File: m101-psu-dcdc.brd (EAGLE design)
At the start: 100 x 50 mm, 49 parts, among them U1 SCREW-M2X8, U2 SCREW-M2X8, U3 NUT-M2-SELFLOCK, U4 NUT-M2-SELFLOCK, U5 FX2-20P-1.27DS, U6 SHHN000A3CL41Z, U7 G3VM-62C1, U8 ERM1-5MM

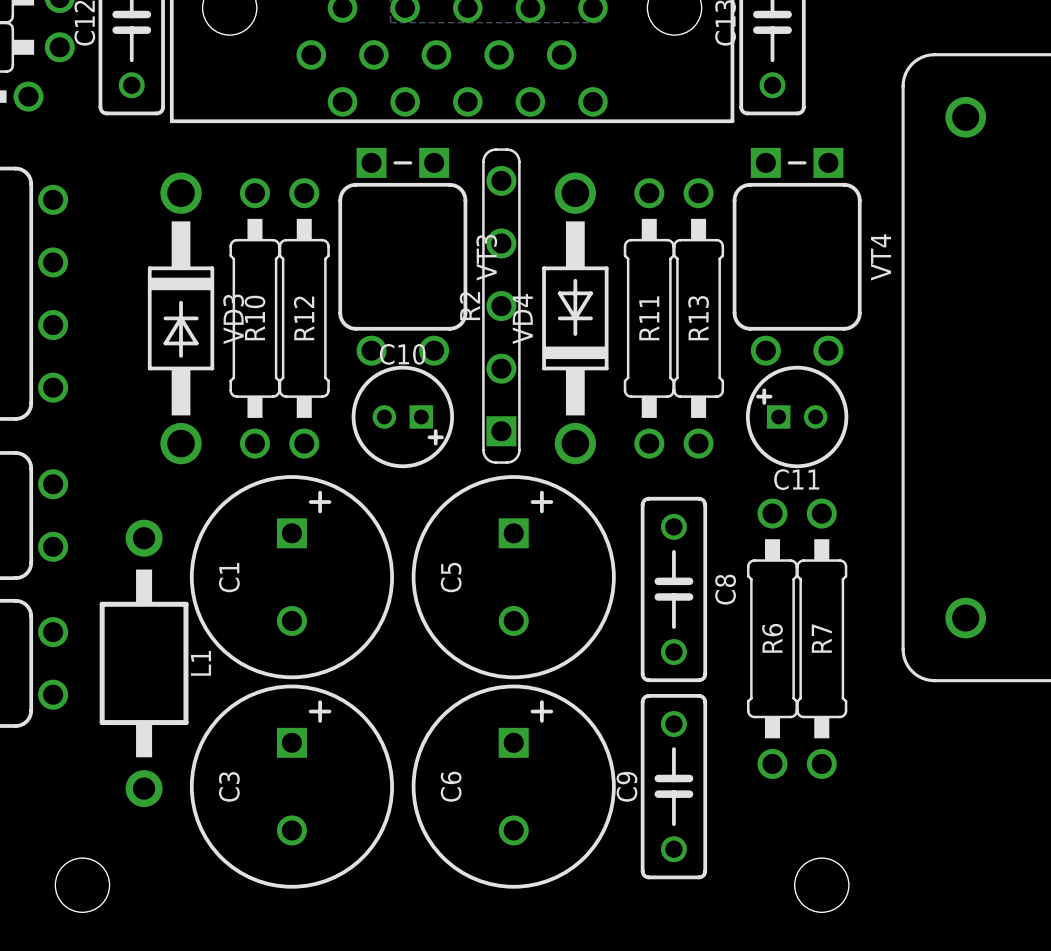
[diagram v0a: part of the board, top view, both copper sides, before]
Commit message: M101c Update
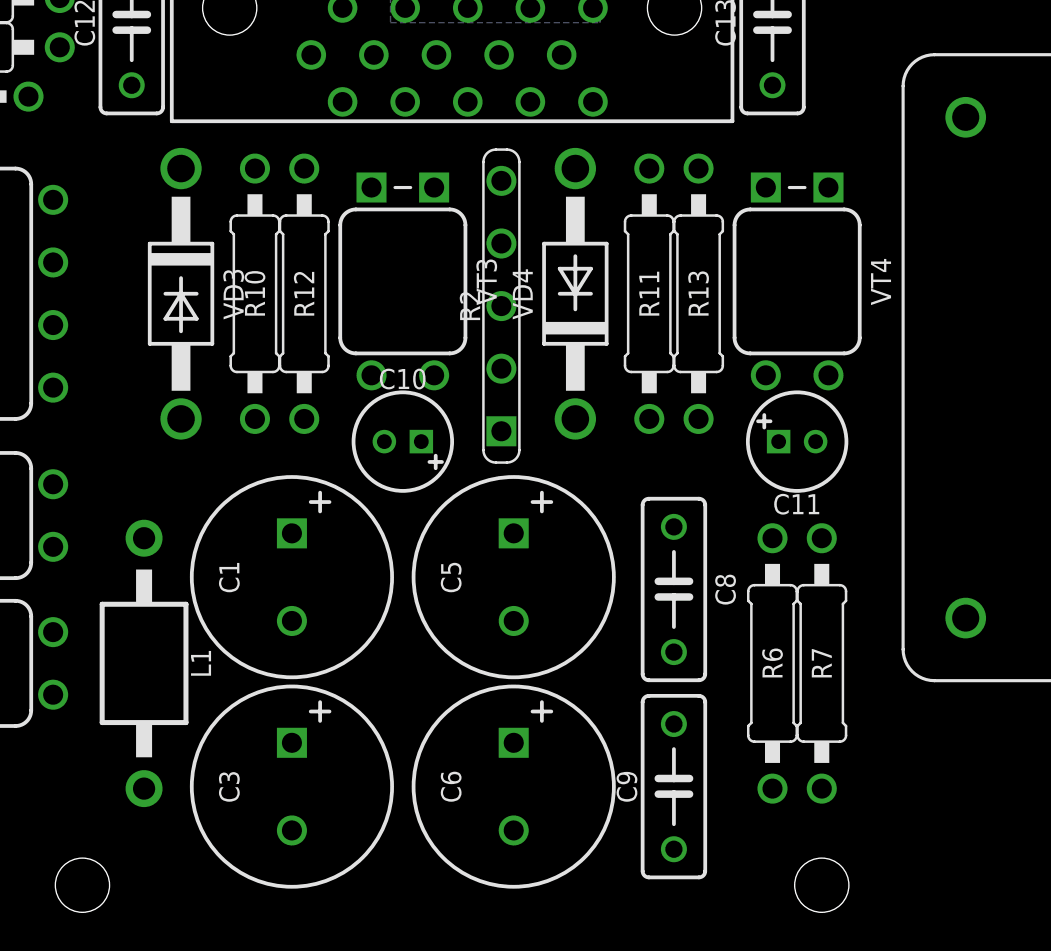
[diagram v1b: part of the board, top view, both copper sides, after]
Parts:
- moved C10 1.00 mm to (48.0, 22.0)
- moved C11 1.00 mm to (64.0, 22.0)
- moved R10 1.00 mm to (42.0, 28.0)
- moved R11 1.00 mm to (58.0, 28.0)
- moved R12 1.00 mm to (44.0, 28.0)
- moved R13 1.00 mm to (60.0, 28.0)
- moved R6 1.00 mm to (63.0, 13.0)
- moved R7 1.00 mm to (65.0, 13.0)
- moved VD3 1.00 mm to (39.0, 28.0)
- moved VD4 1.00 mm to (55.0, 28.0)
- moved VT3 1.00 mm to (48.0, 28.5)
- moved VT4 1.00 mm to (64.0, 28.5)
